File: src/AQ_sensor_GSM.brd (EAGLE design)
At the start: 110 x 64 mm, 113 parts, among them J1 F-1X03-SIP-100-32, J2 53261-0871, J3 PJ-002BH, Q2 MMBT2222, Q3 MMBT2222, Q4 MMBT2222, Q5 MMBT2222, Q6 MMBT2222, Q7 MMBT2222, U3 TEXAS_INSTRUMENTS_LM1117IMP-3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, U5 TXS0108EPWR

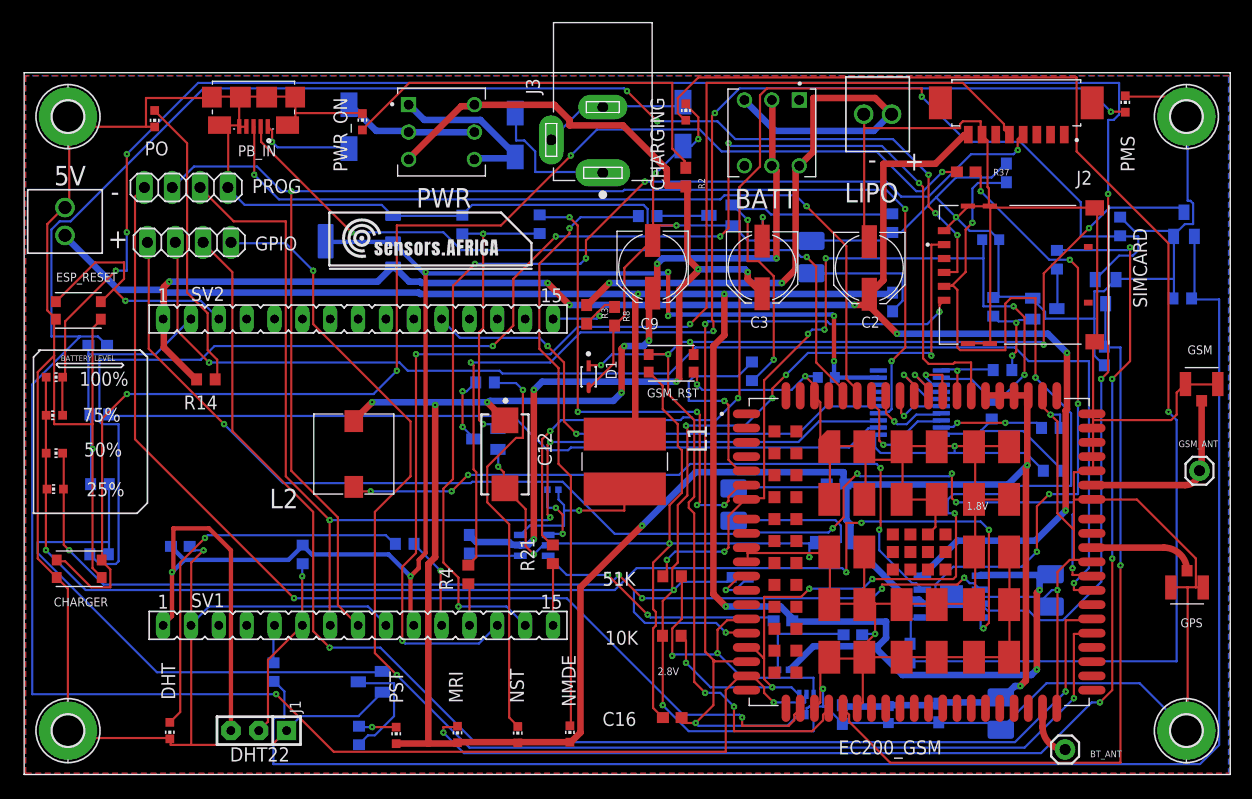
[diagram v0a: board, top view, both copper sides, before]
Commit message: Routed - Minus DW01
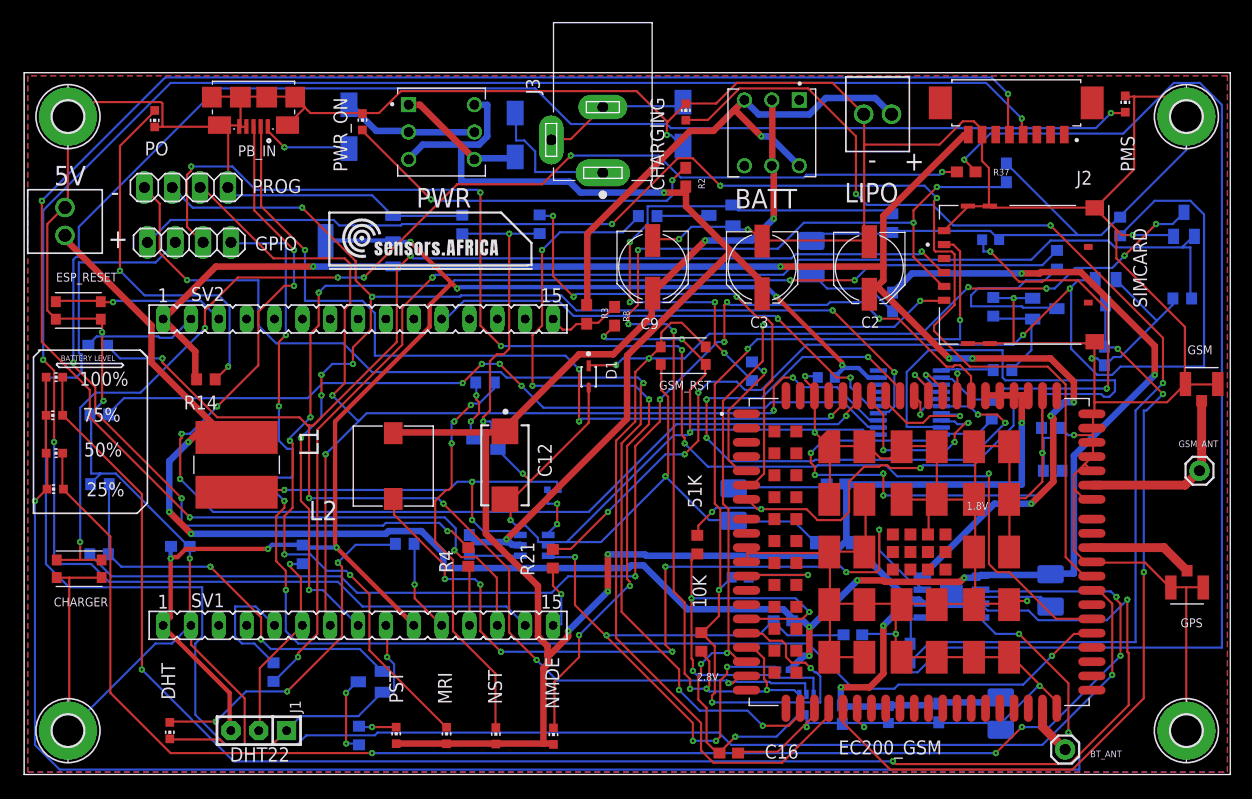
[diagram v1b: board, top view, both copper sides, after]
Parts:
- moved L1 35.4 mm to (19.6, 27.9)
- moved C16 6.09 mm to (64.5, 1.63), turned to 0 degrees
- moved L2 3.76 mm to (33.9, 27.8)
- moved 51K 3.69 mm to (61.7, 20.6), turned to 90 degrees
- moved 10K 2.75 mm to (62.0, 11.8), turned to 90 degrees
- moved NST 2.00 mm to (43.3, 3.21)
- moved R4 1.60 mm to (40.8, 19.5)
- moved NMDE 1.51 mm to (48.5, 3.17)
- moved GSM_RST 1.30 mm to (60.4, 37.9)
- moved MRI 1.00 mm to (38.8, 3.23)
- moved C12 1.00 mm to (44.1, 27.9)
- moved R21 0.40 mm to (48.5, 19.4)
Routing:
- net PMS_TX: track 97.4 -> 174.9 mm, vias 5 -> 3
- net SIMRST: track 230.2 -> 156.6 mm
- net N$4: track 101.6 -> 161.7 mm
- net GND: track 906.5 -> 849.0 mm, vias 18 -> 25
- net MAIN_DTR: track 5.77 -> 60.6 mm, vias 1 -> 5
- net N$45: track 60.8 -> 115.2 mm, vias 5 -> 1
- net PMS_RX: track 114.7 -> 167.7 mm, vias 3 -> 4
- net G_ADC1: track 117.5 -> 164.4 mm, vias 2 -> 1
- net N$17: track 96.2 -> 140.0 mm
- net V_LIPO: track 238.4 -> 205.5 mm, vias 11 -> 8
- net N$40: track 9.52 -> 41.7 mm, vias 2 -> 0
- net N$31: track 14.2 -> 45.5 mm, vias 0 -> 4
- net G_USB_D+: track 75.6 -> 106.8 mm, vias 2 -> 6
- net PWRSTAT: track 138.4 -> 107.8 mm
- net N$18: track 179.6 -> 150.0 mm, vias 5 -> 3
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
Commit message: JLCPCB V2
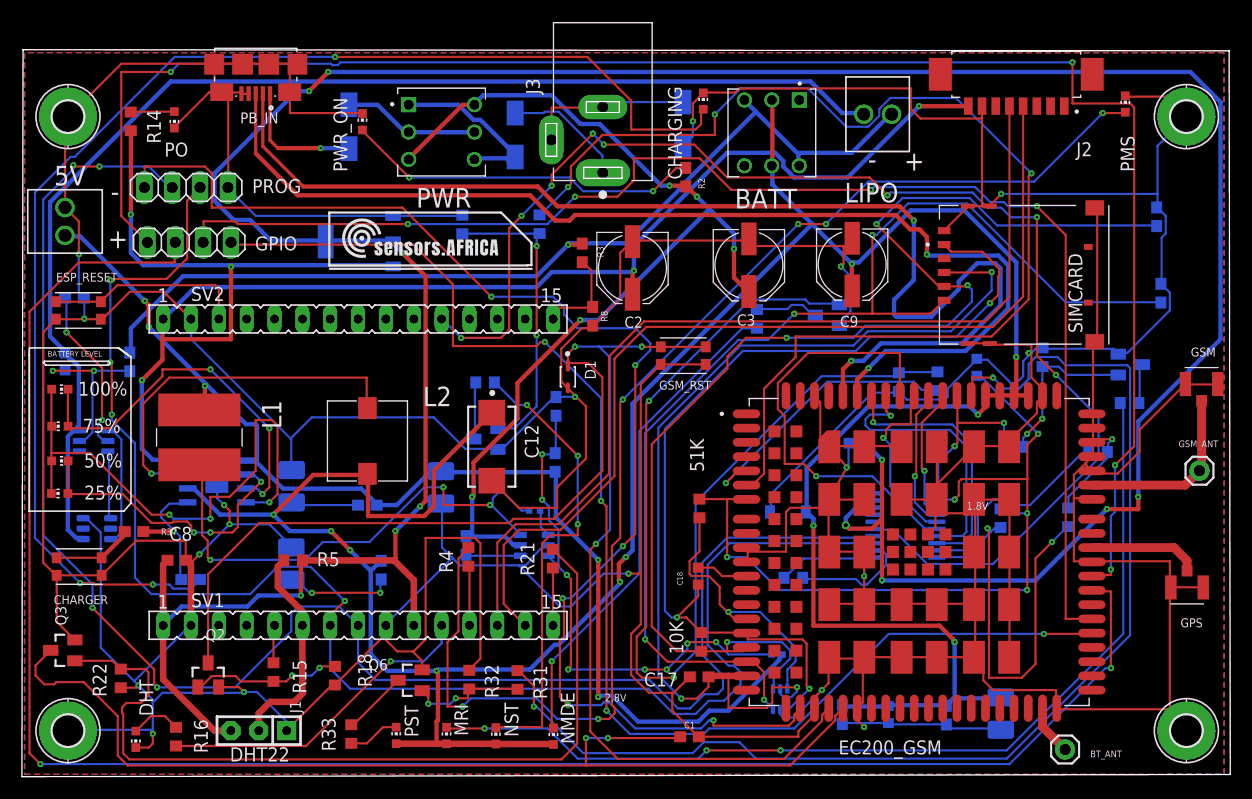
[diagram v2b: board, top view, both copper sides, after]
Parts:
- removed U$2: (no value), IP5306:SOIC127P600X165-9T209N
- added C4: 100nf, 06035C104K4T2A:CAPC1608X90N
- added DW01: DW01-P, DW01-P:SOT23-6L
- added IP5306: IP5306, IP5306:SOIC127P600X165-9T209N
- added Q8: FS8205, FS8205:SOT95P280X145-6N
- added R10: 100R, SparkFun-Resistors:0603
- added R9: 1k, SparkFun-Resistors:0603
- R16, R4: value 470 -> 470R
- R6: value 15 -> 15k
- moved Q3 100.6 mm to (3.79, 11.0), flipped to the top, turned to 90 degrees
- moved R22 100.0 mm to (9.08, 8.44), flipped to the top, turned to 90 degrees
- moved Q2 98.0 mm to (17.0, 8.75), flipped to the top
- moved R18 84.6 mm to (28.6, 8.69), flipped to the top, turned to 90 degrees
- moved R37 82.7 mm to (10.3, 21.8)
- moved R20 66.0 mm to (15.5, 17.5), turned to 0 degrees
- moved R29 65.0 mm to (70.4, 17.6)
- moved C17 62.6 mm to (61.8, 8.58), flipped to the top, turned to 180 degrees
- moved C16 57.5 mm to (103.9, 43.6), flipped to the bottom, turned to 90 degrees
- moved C30 56.4 mm to (38.3, 25.9)
- moved C23 51.8 mm to (24.7, 26.0)
- moved R17 51.4 mm to (31.6, 24.2), turned to 180 degrees
- moved C1 51.4 mm to (60.9, 3.12), flipped to the top, turned to 0 degrees
- moved R19 42.2 mm to (32.8, 18.3), turned to 90 degrees
- moved C24 40.7 mm to (24.6, 18.9), turned to 90 degrees
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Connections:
- new net BATT-: C4.2, DW01.6, LIPO.2, Q8.1
- new net N$19: DW01.3, Q8.4
- new net N$37: C4.1, DW01.5, R10.1
- new net N$47: DW01.2, R9.1
- new net N$9: DW01.1, Q8.6
- net 5V_IN: now also IP5306.1; no longer U$2.1
- net 5V_OUT: now also IP5306.8; no longer U$2.8
- net GND: now also IP5306.9, Q8.3, R9.2; no longer LIPO.2, U$2.9
- net LBV: now also R10.2
- net N$14: now also IP5306.4; no longer U$2.4
- net N$17: now also IP5306.2; no longer U$2.2
- net N$18: now also IP5306.3; no longer U$2.3
- net N$21: now also IP5306.7; no longer U$2.7
- net N$45: now also IP5306.5; no longer U$2.5
- net V_LIPO: now also IP5306.6; no longer U$2.6
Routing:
- net +3V3: track 131.1 -> 286.9 mm, vias 7 -> 11
- net N$18: track 150.0 -> 34.7 mm
- net BATT-: track 0.00 -> 113.7 mm
- net N$17: track 140.0 -> 27.2 mm, vias 5 -> 3
- net N$1: track 119.9 -> 13.7 mm
- net N$45: track 115.2 -> 12.6 mm
- net N$20: track 109.5 -> 7.36 mm, vias 6 -> 0
- net N$14: track 149.1 -> 49.9 mm
- net GND: track 849.0 -> 947.9 mm, vias 25 -> 19
- net PMS_TX: track 174.9 -> 88.5 mm, vias 3 -> 0
- net PMS_RX: track 167.7 -> 87.2 mm, vias 4 -> 0
- net 5V_IN: track 184.6 -> 105.8 mm, vias 9 -> 5
- net MCU_DTR: track 45.0 -> 122.2 mm, vias 2 -> 8
- net SIMRST: track 156.6 -> 87.9 mm, vias 7 -> 3
- net V_LIPO: track 205.5 -> 272.0 mm, vias 8 -> 11
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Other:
- board size 110 x 64 mm -> 110.2 x 66.3 mm
